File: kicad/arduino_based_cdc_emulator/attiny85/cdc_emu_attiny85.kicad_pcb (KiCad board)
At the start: 2 copper layers, 15.6 x 13 mm, 12 parts, among them IC1 ATTINY85-S, P1 CONN_01X05, P2 CONN_01X03, U1 AP1117D50, U2 LM78L05ACZ

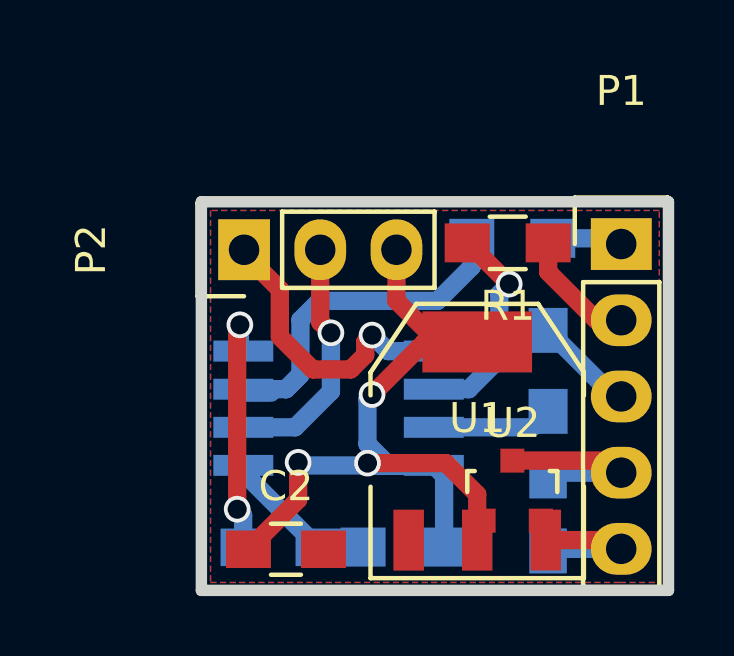
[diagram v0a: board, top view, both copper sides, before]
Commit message: updates
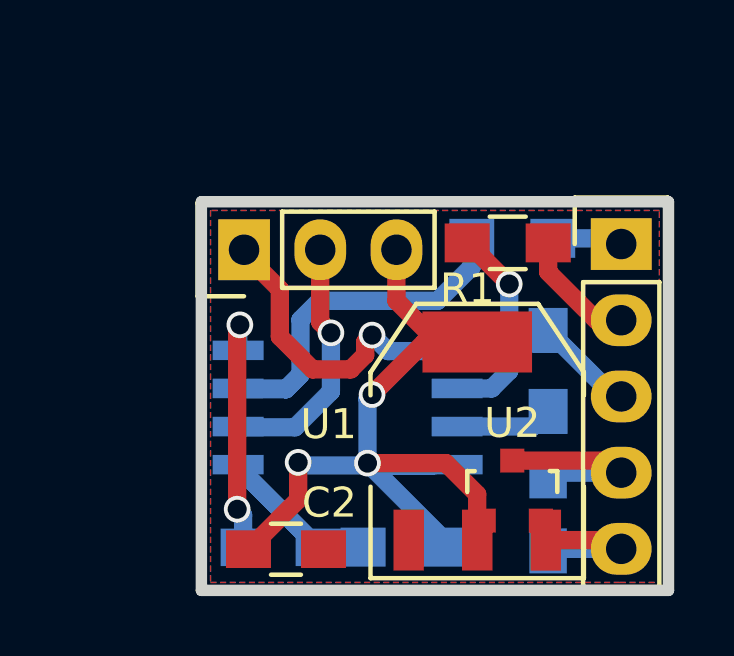
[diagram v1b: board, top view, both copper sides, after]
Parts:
- IC1: footprint my_modules:SOIC-8-N_wide_pads -> Housings_SOIC.pretty:SOIJ-8_5.3x5.3mm_Pitch1.27mm
- moved IC1 0.31 mm to (182.9, 98.9), turned to 0 degrees
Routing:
- net Net-(C3-Pad1): track 5.20 -> 9.06 mm
- net +5V: track 33.0 -> 32.1 mm
- net Net-(IC1-Pad3): track 13.0 -> 13.6 mm
